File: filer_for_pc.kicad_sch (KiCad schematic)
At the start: 43 parts

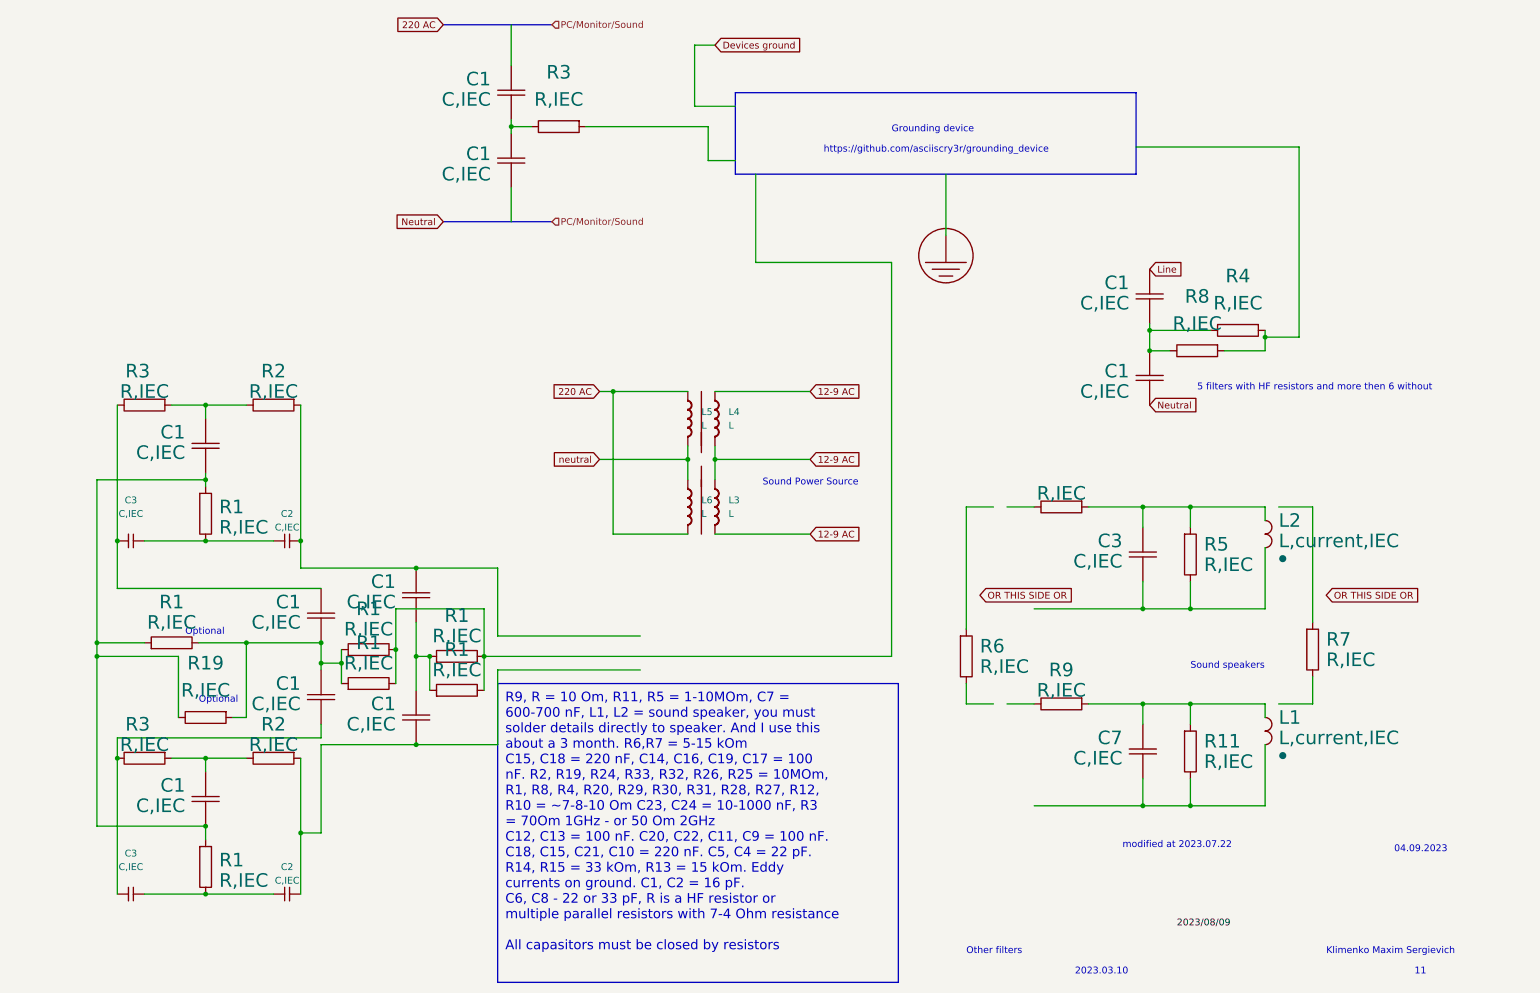
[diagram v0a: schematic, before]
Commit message: Upgrade
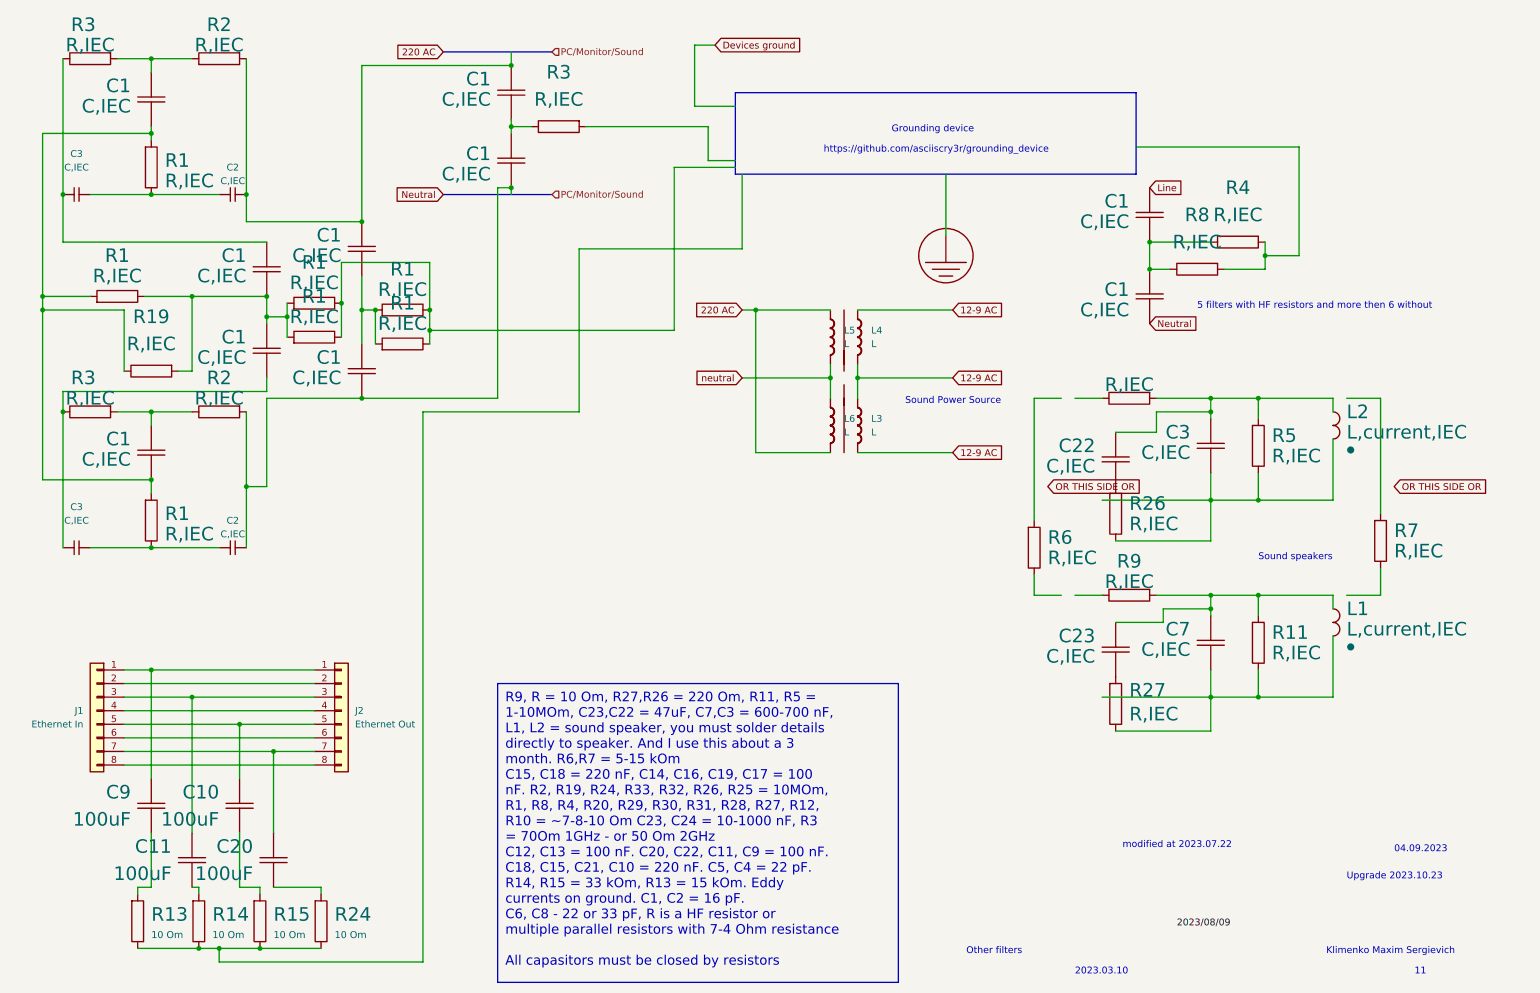
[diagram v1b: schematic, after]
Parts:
- added C10, C11, C20, C9: 100uF, symbol PCM_Generic:C,IEC
- added C22, C23: C,IEC, symbol PCM_Generic:C,IEC
- added J1: Ethernet In, 4ms_Connector:Pins_1x08_2.54mm_TH, symbol PCM_4ms_Connector:Conn_01x08
- added J2: Ethernet Out, 4ms_Connector:Pins_1x08_2.54mm_TH, symbol PCM_4ms_Connector:Conn_01x08
- added R13, R14, R15, R24: 10 Om, symbol PCM_Generic:R,IEC
- added R26, R27: R,IEC, symbol PCM_Generic:R,IEC
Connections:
- net at C7.1 (+), L1.1 (+), R11.1 (+)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: now also C23.1 (+)
- net at C7.2 (-), L1.2 (-), R11.2 (-): now also R27.2 (-)
- net at C3.1 (+), L2.1 (+), R2.1 (+)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: now also C22.1 (+)
- net at C3.2 (-), L2.2 (-), R5.2 (-): now also R26.2 (-)
- net at C1.1 (+), C2.1 (+), R2.1 (+): now also C1.1 (+)
- net at C1.2 (-), C2.1 (+), R2.1 (+): now also C1.2 (-)
- new net: C9.1 (+), J1.1 (Pin_1), J2.1 (Pin_1)
- new net: C9.2 (-), R13.1 (+)
- new net: C10.1 (+), J1.5 (Pin_5), J2.5 (Pin_5)
- new net: C10.2 (-), R15.1 (+)
- new net: C22.2 (-), R26.1 (+)
- new net: R13.2 (-), R14.2 (-), R15.2 (-), R24.2 (-)
- new net: J1.2 (Pin_2), J2.2 (Pin_2)
- new net: C11.1 (+), J1.3 (Pin_3), J2.3 (Pin_3)
- new net: J1.4 (Pin_4), J2.4 (Pin_4)
- new net: J1.6 (Pin_6), J2.6 (Pin_6)
- new net: C20.1 (+), J1.7 (Pin_7), J2.7 (Pin_7)
- new net: J1.8 (Pin_8), J2.8 (Pin_8)
- new net: C11.2 (-), R14.1 (+)
- new net: C20.2 (-), R24.1 (+)
- new net: C23.2 (-), R27.1 (+)
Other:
- note added: "Upgrade 2023.10.23"
- note removed: "Optional"
- moved on the sheet: C1, C2, C3, C7, L1, L2, L3, L4, L5, L6, R1, R11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

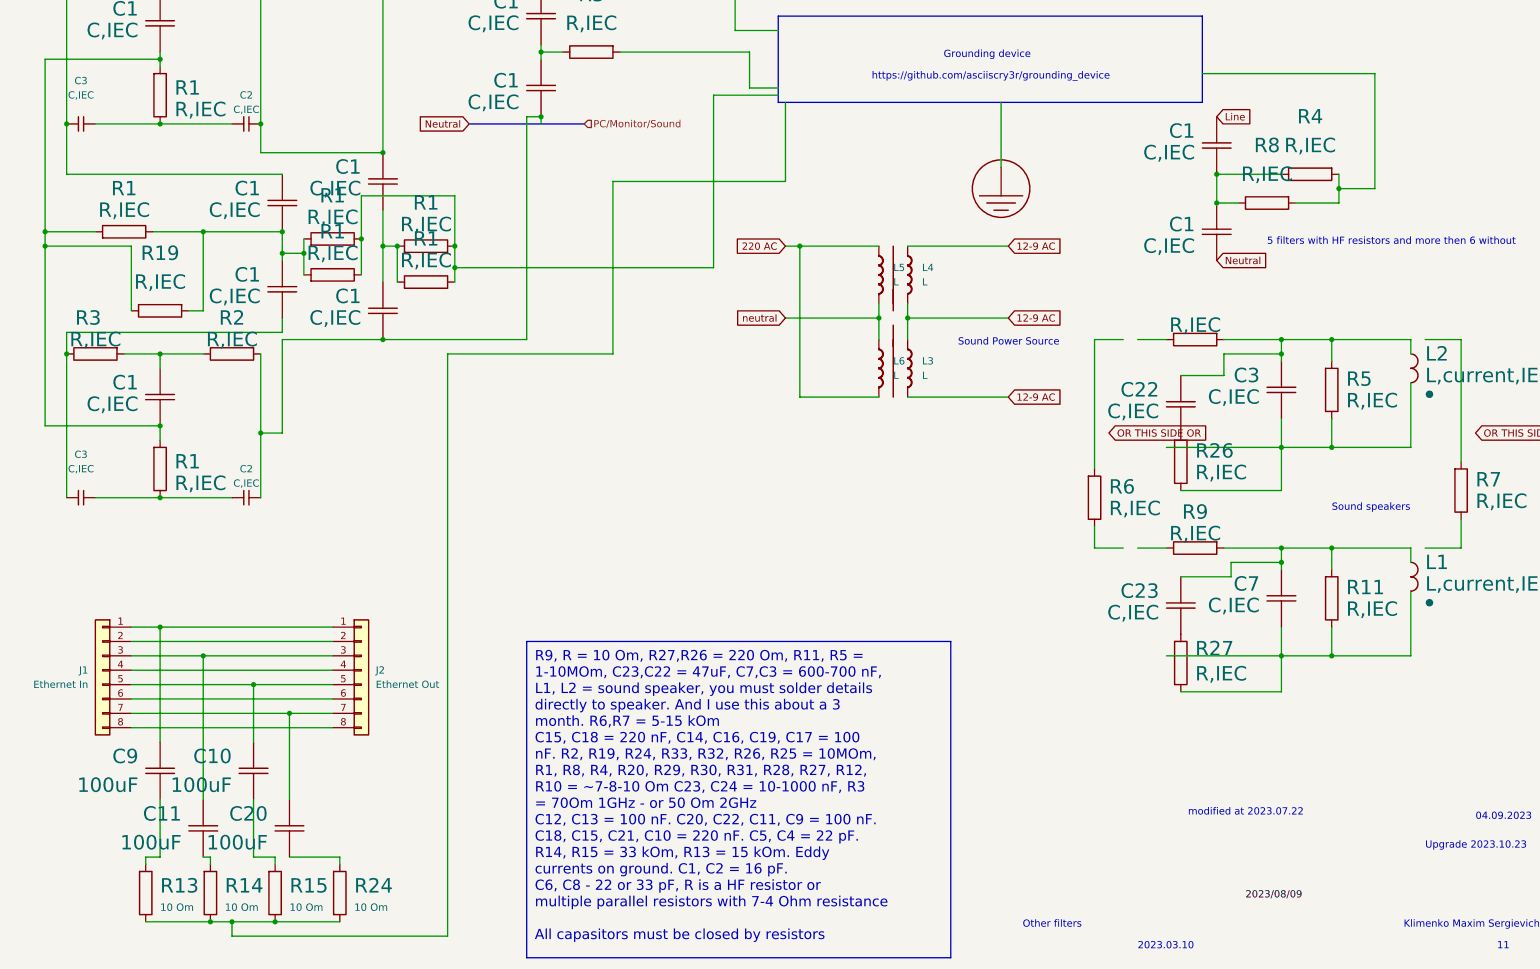
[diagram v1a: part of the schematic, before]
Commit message: Upgrade
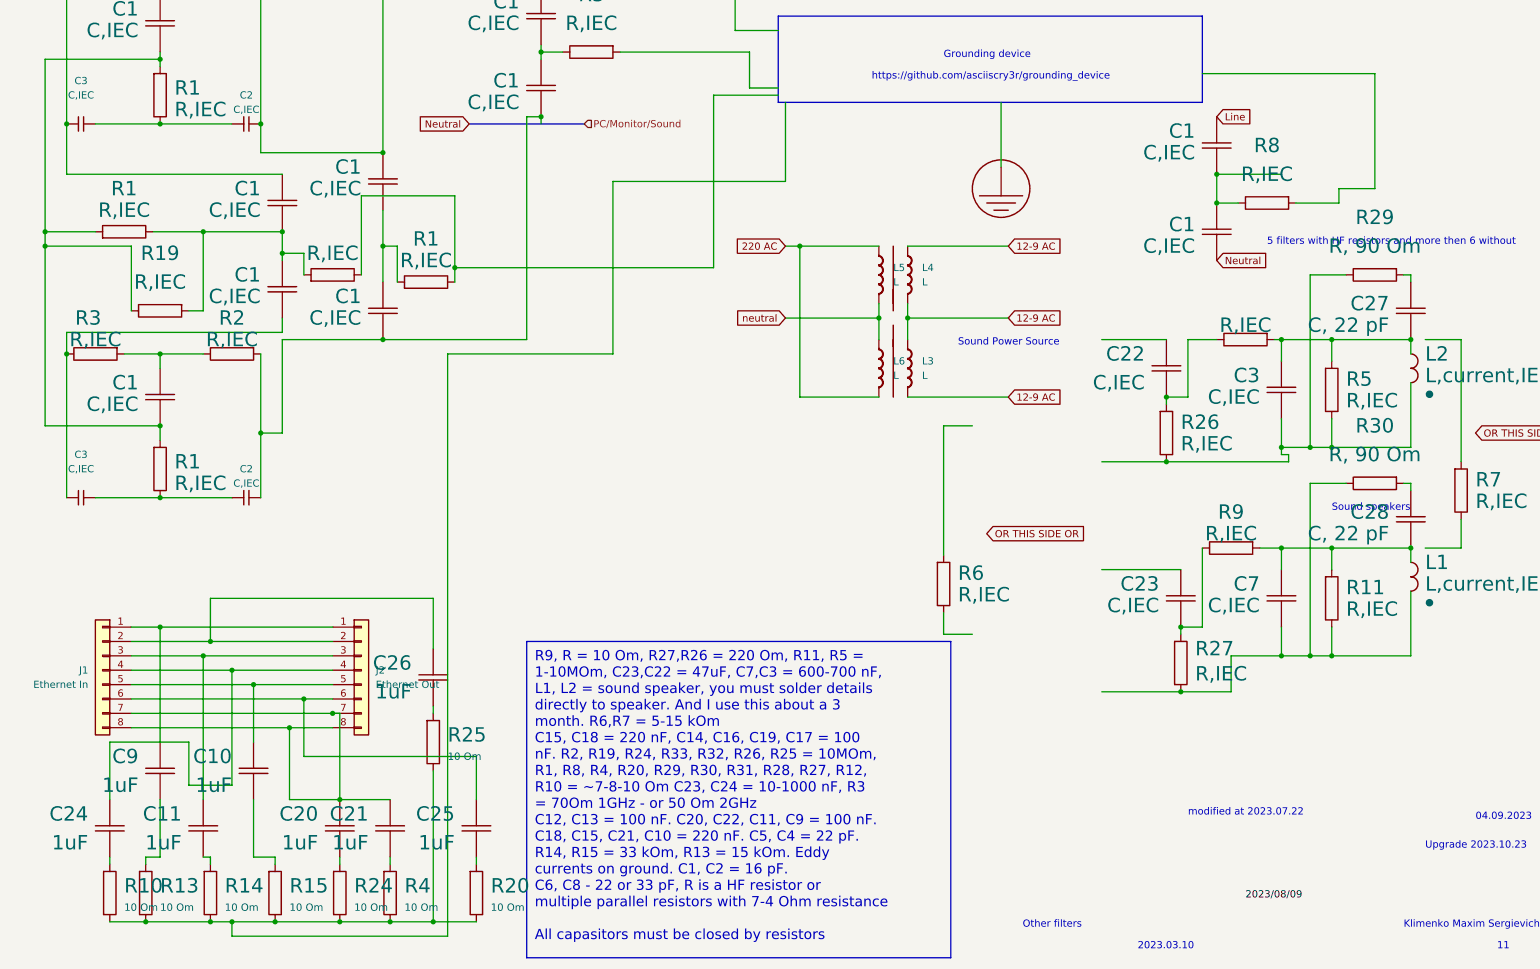
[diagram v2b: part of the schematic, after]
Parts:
- removed R1 (x2): R,IEC, symbol PCM_Generic:R,IEC
- added C21, C24, C25, C26: 1uF, symbol PCM_Generic:C,IEC
- added C27, C28: C, 22 pF, symbol PCM_Generic:C,IEC
- added R10, R20, R25: 10 Om, symbol PCM_Generic:R,IEC
- added R29, R30: R, 90 Om, symbol PCM_Generic:R,IEC
- C10, C11, C20, C9: value 100uF -> 1uF
- R4: value R,IEC -> 10 Om
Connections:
- net at C7.1 (+), L1.1 (+), R11.1 (+)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: now also C28.2 (-); no longer C23.1 (+)
- net at C7.2 (-), L1.2 (-), R11.2 (-)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: now also R30.2 (-)
- net at C3.1 (+), L2.1 (+), R2.1 (+)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: now also C27.2 (-); no longer C22.1 (+)
- net at C3.2 (-), L2.2 (-), R26.2 (-)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: now also R29.2 (-)
- net at R9.2 (-): now also C23.2 (-), R27.1 (+)
- net at C22.2 (-), R26.1 (+): now also R2.2 (-)
- net at C1.1 (+), C1.2 (-), R8.2 (-): no longer R4.2 (-)
- net at R13.2 (-), R14.2 (-), R15.2 (-)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: now also R4.2 (-), R10.2 (-), R20.2 (-), R25.2 (-)
- net at J1.2 (Pin_2), J2.2 (Pin_2): now also C26.1 (+)
- net at J1.4 (Pin_4), J2.4 (Pin_4): now also C24.1 (+)
- net at J1.6 (Pin_6), J2.6 (Pin_6): now also C25.1 (+)
- net at C20.1 (+), J1.7 (Pin_7), J2.7 (Pin_7): now also J1.8 (Pin_8), J2.8 (Pin_8), C21.1 (+)
- net at R4.1 (+): now also C21.2 (-); no longer R8.1 (+)
- new net: C25.2 (-), R20.1 (+)
- new net: C28.1 (+), R30.1 (+)
- new net: C24.2 (-), R10.1 (+)
- new net: C26.2 (-), R25.1 (+)
- new net: C27.1 (+), R29.1 (+)
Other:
- moved on the sheet: C20, C22, C23, R26, R6, R9

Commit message: Upgrade
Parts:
- removed C10, C11, C20, C21, C24, C25, C9: 1uF, symbol PCM_Generic:C,IEC
- removed L3, L4, L5, L6: L, symbol PCM_Elektuur:L
- added C10, C11, C20, C21, C24, C25, C29, C9: ~50uF, symbol PCM_Elektuur:C-polar
- added C30, C41, C43: C, 100 nF, symbol PCM_Generic:C,IEC
- added C31, C32, C34, C39, C47, C48: C, 22 pF, symbol PCM_Generic:C,IEC
- added C33, C40: C, 10 nF, symbol PCM_Generic:C,IEC
- added C35, C38, C42, C44: C,1uF, symbol PCM_Generic:C,IEC
- added C36, C37, C45, C46: C,680pF, symbol PCM_Generic:C,IEC
- added L3: L,Sound speaker L, symbol PCM_Generic:L,current,IEC
- added L4: L, Sound speaker R, symbol PCM_Generic:L,current,IEC
- added L5: L, Sound speaker L, symbol PCM_Generic:L,current,IEC
- added L6: L,Sound speaker R, symbol PCM_Generic:L,current,IEC
- added R31, R32, R33, R34, R36, R43, R45, R46, R53: R, 10 Om, symbol PCM_Generic:R,IEC
- added R35, R52: R, 90 Om, symbol PCM_Generic:R,IEC
- added R37, R42, R44: R,10KoM, symbol PCM_Generic:R,IEC
- added R38: R, 10 MOM, symbol PCM_Generic:R,IEC
- added R39, R50: R,10Om, symbol PCM_Generic:R,IEC
- added R40, R48: R,10 Om, symbol PCM_Generic:R,IEC
- added R41, R49: R,10MoM, symbol PCM_Generic:R,IEC
- added R47: R,10 KoM, symbol PCM_Generic:R,IEC
- added R51: R,10 MOM, symbol PCM_Generic:R,IEC
- C26: value 1uF -> C, 100 nF
- L1: value L,current,IEC -> L, Sound speaker
- L2: value L,current,IEC -> L,Sound speaker
- R7: value R,IEC -> R, 10 Om
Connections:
- net at C28.2 (-), C7.1 (+), L1.1 (+)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: now also C32.1 (+)
- net GND: now reaches C7.2 (-), L1.2 (-), R11.2 (-), R27.2 (-), R30.2 (-)
- net GND: now also C26.2 (-), C3.2 (-), L2.2 (-), R26.2 (-), R29.2 (-), R5.2 (-), R7.2 (-), C30.2 (-), R33.2 (-)
- net at C27.2 (-), C3.1 (+), L2.1 (+)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: now also C31.2 (-)
- net at J1.6 (Pin_6), J2.6 (Pin_6): now also C10.2 (-)
- net at R20.1 (+): now also C10.1 (+)
- net at J1.1 (Pin_1), J2.1 (Pin_1): now also C20.1 (+)
- net at R13.1 (+): now also C20.2 (-)
- net at R7.1 (+): now also C31.1 (+)
- net at J1.5 (Pin_5), J2.5 (Pin_5): now also C21.1 (+)
- net at R15.1 (+): now also C21.2 (-)
- net at C22.1 (+): now also R6.1 (+), R32.1 (+)
- net at R10.1 (+): now also C29.2 (-)
- net at C1.1 (+), C1.2 (-): now also R8.1 (+); no longer R8.2 (-)
- net at R25.1 (+): now also C25.1 (+); no longer C26.2 (-)
- net at J1.2 (Pin_2), J2.2 (Pin_2): now also C25.2 (-); no longer C26.1 (+)
- net at J1.4 (Pin_4), J2.4 (Pin_4): now also C24.2 (-)
- net at R4.1 (+): now also C11.1 (+)
- net at J1.3 (Pin_3), J2.3 (Pin_3): now also C9.1 (+)
- net at J1.7 (Pin_7), J2.7 (Pin_7): now also C29.1 (+); no longer J1.8 (Pin_8), J2.8 (Pin_8)
- net at R14.1 (+): now also C9.2 (-)
- net at R6.2 (-): now also C23.1 (+), R31.1 (+)
- net at R24.1 (+): now also C24.1 (+)
- new net: C36.1 (+), L4.1 (+), R38.1 (+), R39.1 (+)
- new net: C38.2 (-), R39.2 (-), R42.1 (+)
- new net: C39.2 (-), R43.1 (+)
- new net: C35.2 (-), R37.1 (+), R40.2 (-)
- new net: C34.2 (-), C37.2 (-), C39.1 (+), C44.1 (+), L3.2 (-), R34.2 (-), R36.2 (-), R37.2 (-), R41.2 (-)
- new net: C45.1 (+), L5.1 (+), R48.1 (+), R49.1 (+)
- new net: C32.2 (-), R33.1 (+)
- new net: C37.1 (+), L3.1 (+), R40.1 (+), R41.1 (+)
- new net: C44.2 (-), R47.1 (+), R48.2 (-)
- new net: C11.2 (-), J1.8 (Pin_8), J2.8 (Pin_8)
- new net: C47.1 (+), R52.1 (+)
- new net: C38.1 (+), C46.2 (-), C47.2 (-), C48.1 (+), L6.2 (-), R44.2 (-), R45.2 (-), R46.2 (-), R51.2 (-)
- new net: C46.1 (+), L6.1 (+), R50.1 (+), R51.1 (+)
- new net: C40.1 (+), R46.1 (+)
- new net: C41.1 (+), R45.1 (+)
- new net: C42.2 (-), R44.1 (+), R50.2 (-)
- new net: C34.1 (+), R35.1 (+)
- new net: C26.1 (+), R31.2 (-)
- new net: C33.1 (+), R36.1 (+)
- new net: C43.1 (+), R34.1 (+)
- new net: C30.1 (+), R32.2 (-)
- new net: C48.2 (-), R53.1 (+)
- new net GNDA: C33.2 (-), C35.1 (+), C36.2 (-), C40.2 (-), C41.2 (-), C42.1 (+), C43.2 (-), C45.2 (-), L4.2 (-), L5.2 (-), R35.2 (-), R38.2 (-), R42.2 (-), R43.2 (-), R47.2 (-), R49.2 (-), R52.2 (-), R53.2 (-)
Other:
- note added: "1969 PRO JLH Class"
- note removed: "Sound Power Source"
- note removed: "Sound speakers"
- moved on the sheet: C1, C22, C23, C27, C28, C3, C7, L1, L2, R11, R24, R25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
